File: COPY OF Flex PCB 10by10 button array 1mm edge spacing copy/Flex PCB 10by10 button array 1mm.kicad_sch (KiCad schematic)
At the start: 202 parts, among them J1 522071060, J2 522071060

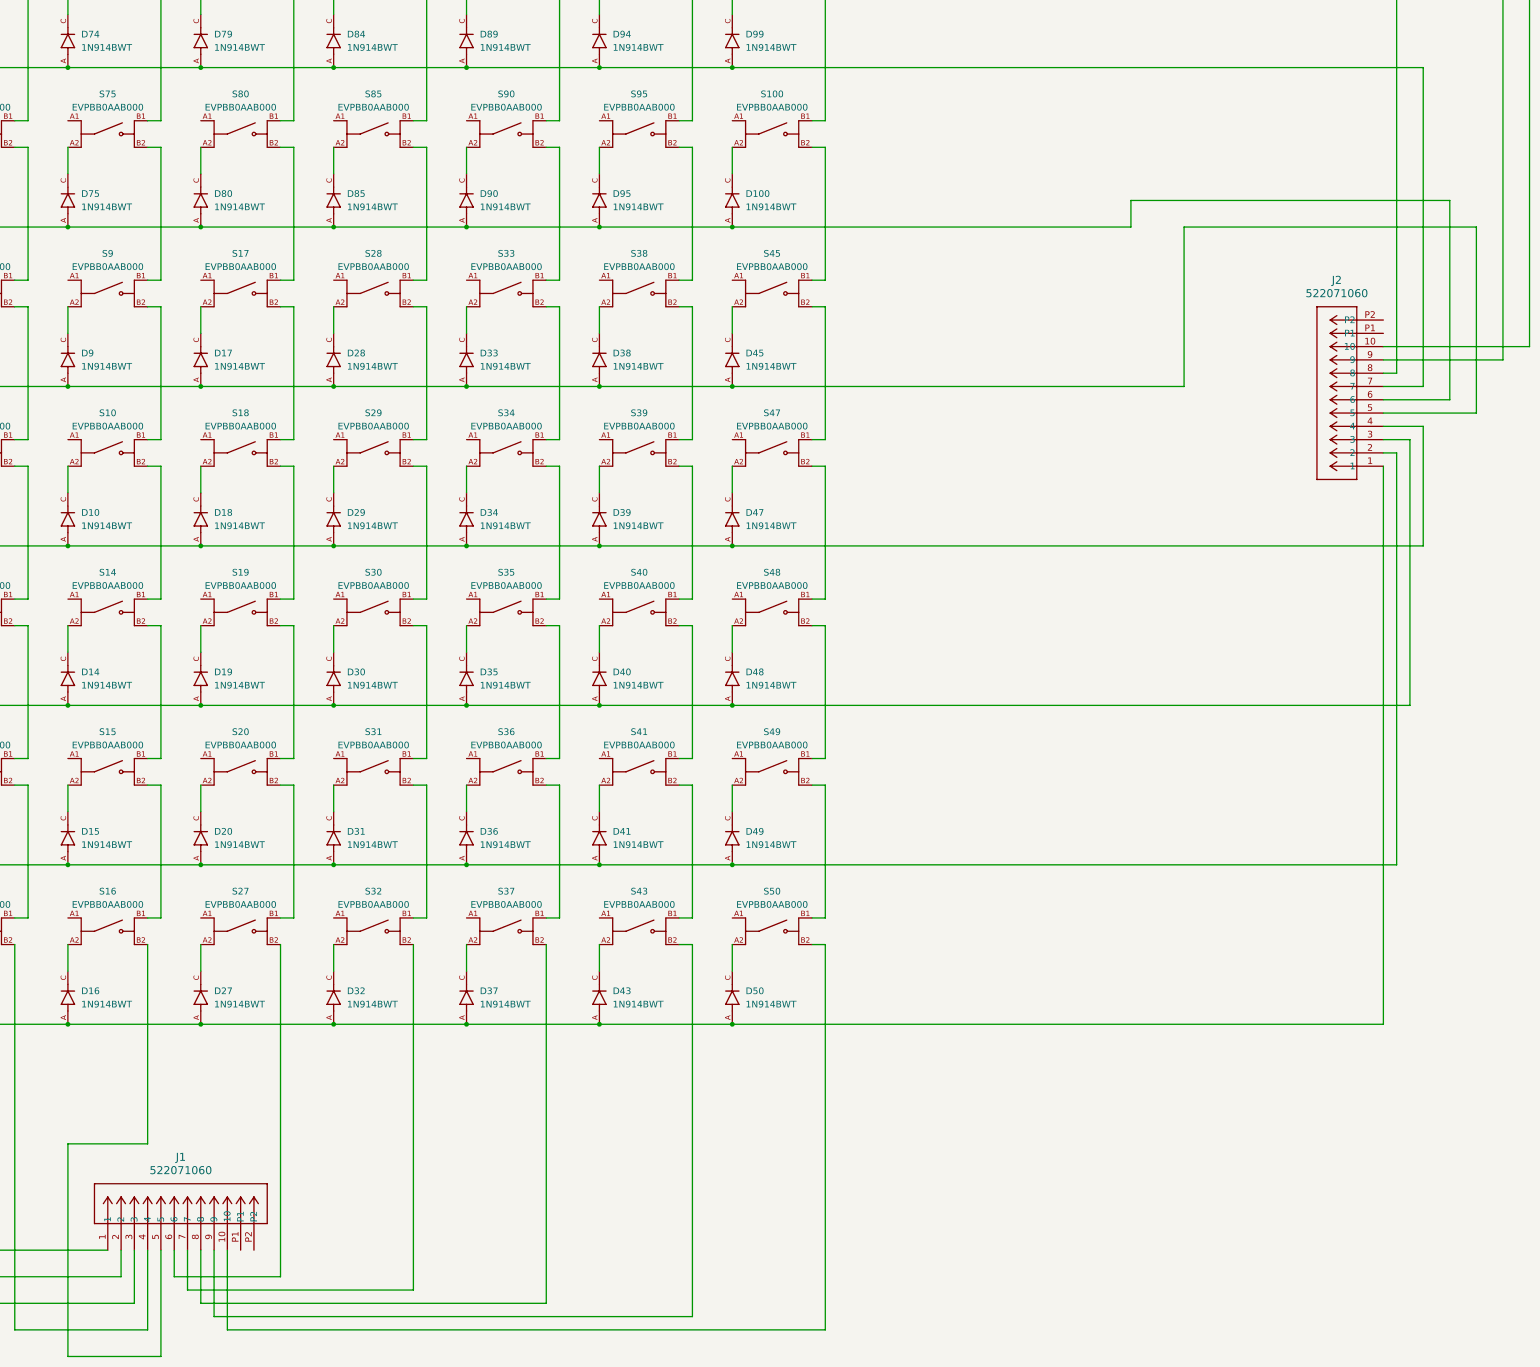
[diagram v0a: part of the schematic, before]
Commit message: Add files via upload
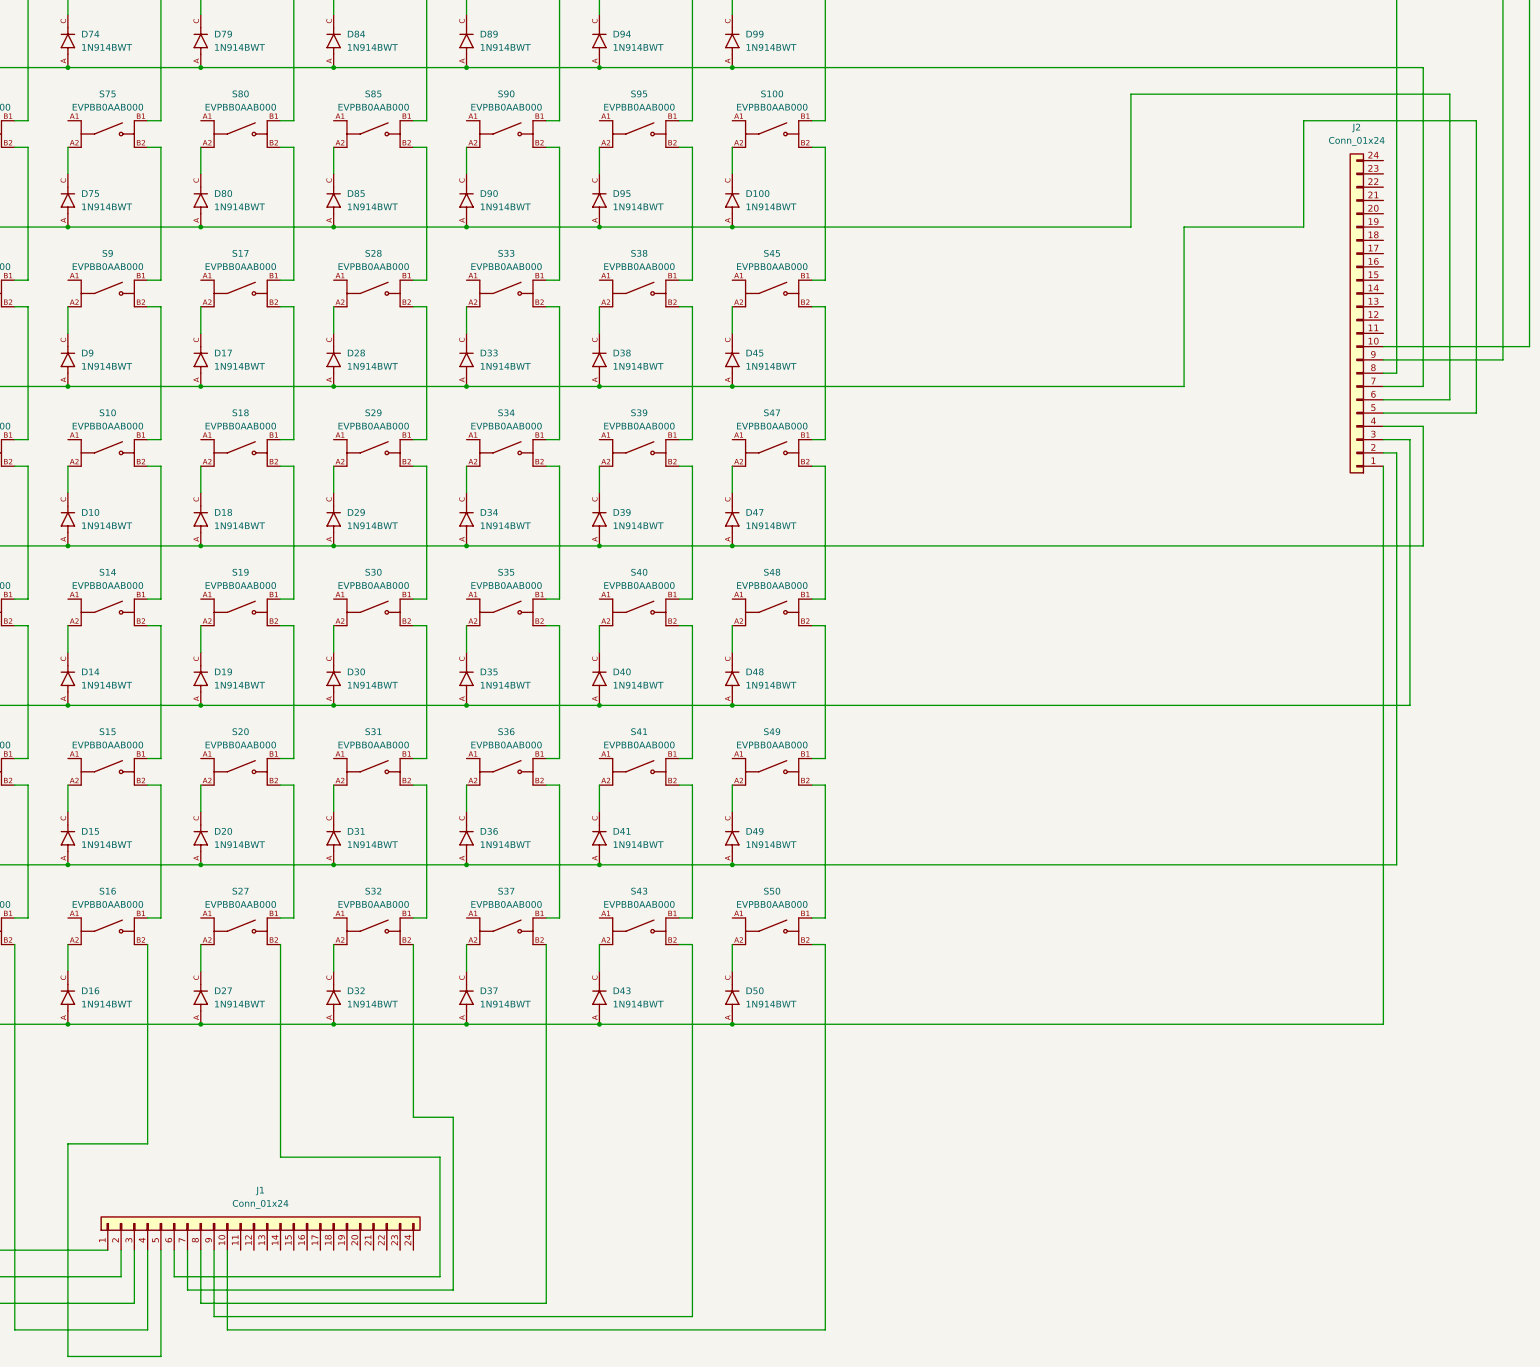
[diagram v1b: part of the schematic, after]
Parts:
- removed J1, J2: 522071060, costumized ffc connector 24pos:customized 24pos connector 1mm pitch footprint, symbol molex connector 10pos 1mm:522071060
- added J1, J2: Conn_01x24, costumized ffc connector 24pos:24pos edge connector, symbol Connector_Generic:Conn_01x24
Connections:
- net at D10.A, D18.A, D21.A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: now also J2.4 (Pin_4)
- net at D1.A, D16.A, D2.A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: now also J2.1 (Pin_1)
- net at D51.A, D56.A, D61.A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: now also J2.10 (Pin_10)
- net at D11.A, D12.A, D13.A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: now also J2.2 (Pin_2)
- net at D14.A, D19.A, D22.A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: now also J2.3 (Pin_3)
- net at D17.A, D28.A, D33.A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: now also J2.5 (Pin_5)
- net at D100.A, D55.A, D60.A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: now also J2.6 (Pin_6)
- net at D54.A, D59.A, D64.A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: now also J2.7 (Pin_7)
- net at D53.A, D58.A, D63.A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: now also J2.8 (Pin_8)
- net at D52.A, D57.A, D62.A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: now also J2.9 (Pin_9)
- net at S32.B2: now also J1.7 (Pin_7)
- net at S50.B2: now also J1.10 (Pin_10)
- net at S27.B2: now also J1.6 (Pin_6)
- net at S37.B2: now also J1.8 (Pin_8)
- net at S1.B2: now also J1.1 (Pin_1)
- net at S8.B2: now also J1.4 (Pin_4)
- net at S43.B2: now also J1.9 (Pin_9)
- net at S2.B2: now also J1.2 (Pin_2)
- net at S3.B2: now also J1.3 (Pin_3)
- net at S16.B2: now also J1.5 (Pin_5)
